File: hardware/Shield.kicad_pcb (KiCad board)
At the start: 2 copper layers, 29 parts, among them IC1 TP4056-42-ESOP8, P1 CONN_14_1, P2 CONN_14_2, SW1 JS202011SCQN

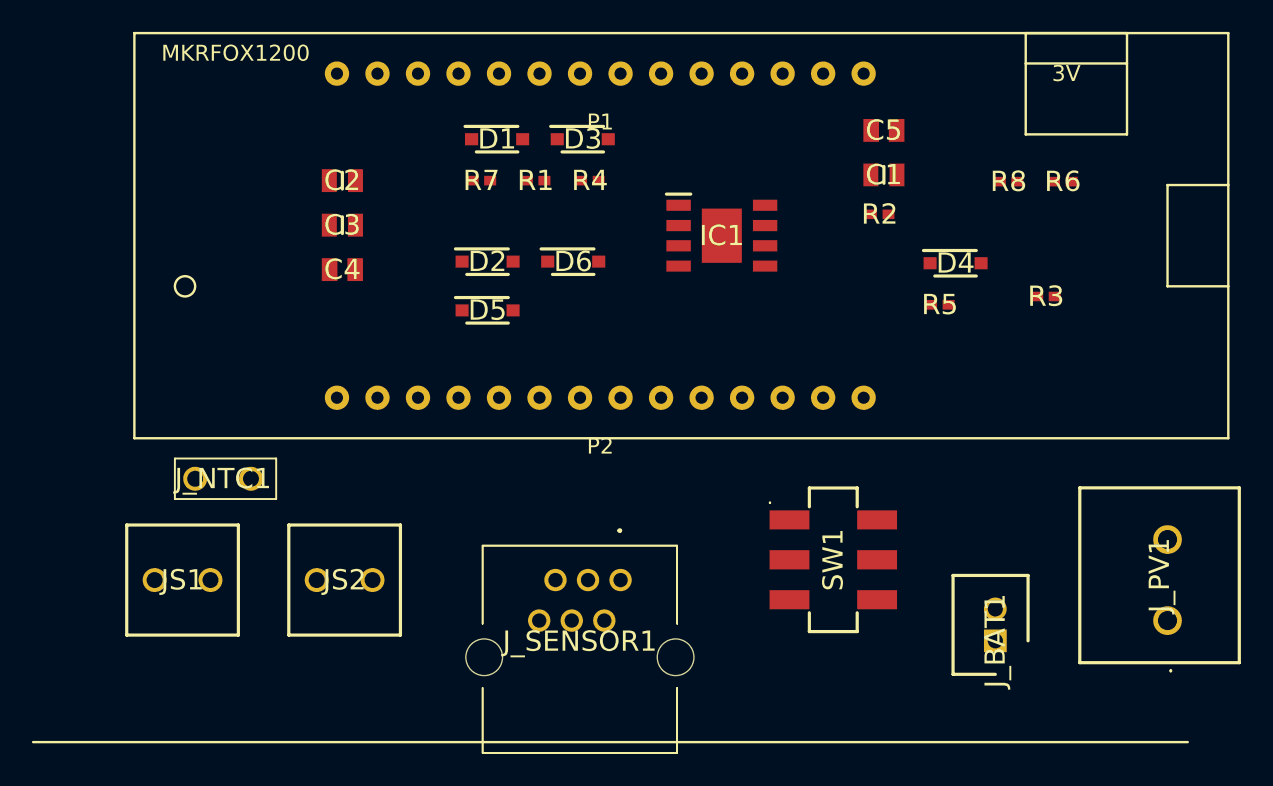
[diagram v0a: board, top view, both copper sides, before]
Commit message: completed PCB, DRC OK
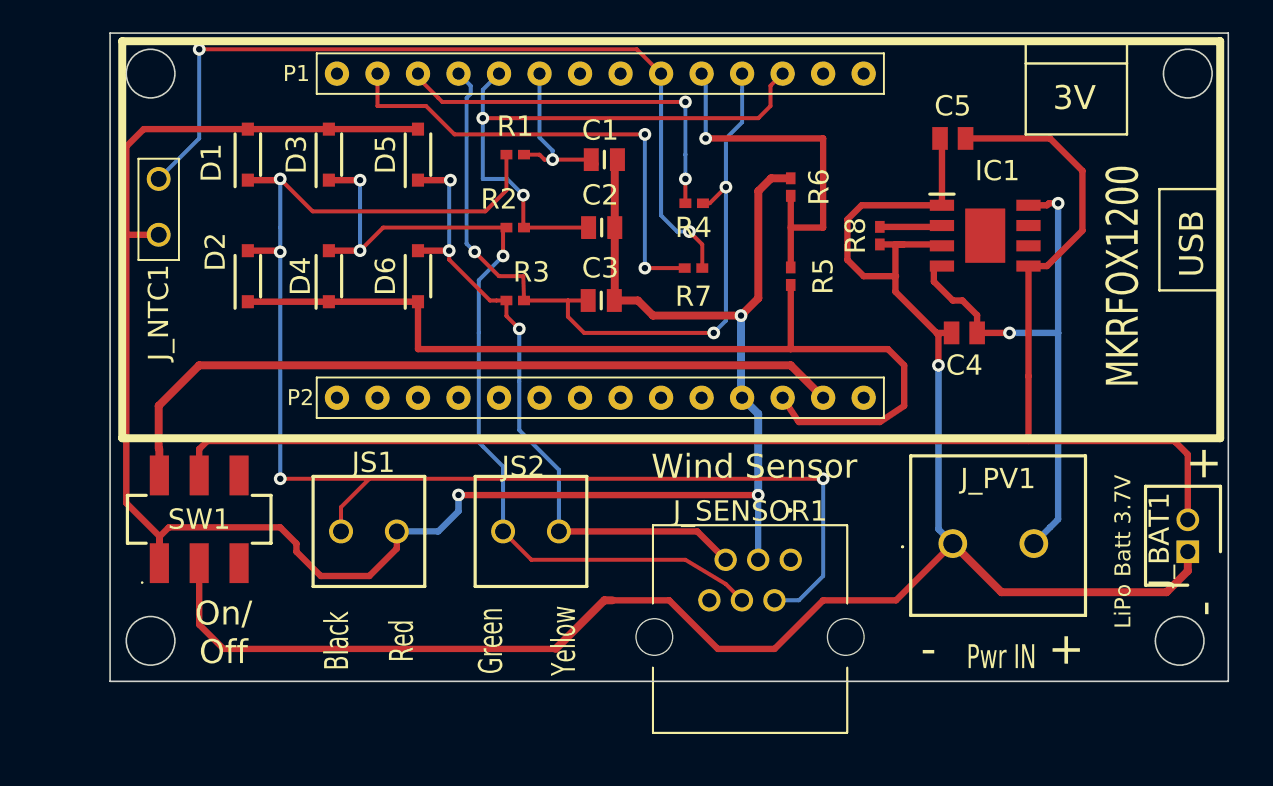
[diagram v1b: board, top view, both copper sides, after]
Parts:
- P1: footprint JLCPCB_FP:CONN14_FP -> JLCPCB_FP:CONN14_FP1
- P2: footprint JLCPCB_FP:CONN14_FP -> JLCPCB_FP:CONN14_FP2
- moved SW1 39.8 mm to (80.3, 96.5), turned to 0 degrees
- moved D4 39.3 mm to (88.4, 81.3), turned to 90 degrees
- moved C4 39.2 mm to (128.2, 84.8)
- moved R3 33.3 mm to (100.1, 82.8)
- moved R2 22.9 mm to (100.1, 78.2)
- moved J_NTC1 18.9 mm to (77.7, 75.2), turned to 270 degrees
- moved C1 17.6 mm to (105.7, 74.0), turned to 180 degrees
- moved R6 17.1 mm to (117.3, 75.7), turned to 90 degrees
- moved C3 16.9 mm to (105.5, 82.8), turned to 180 degrees
- moved C2 16.5 mm to (105.5, 78.2), turned to 180 degrees
- moved IC1 16.5 mm to (129.5, 78.7)
- moved D3 15.9 mm to (88.4, 73.7), turned to 90 degrees
- moved D1 15.7 mm to (83.3, 73.7), turned to 90 degrees
- moved D2 15.1 mm to (83.3, 81.3), turned to 90 degrees
- moved R7 14.4 mm to (111.3, 80.8)
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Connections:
- C1 pad 1: Net-(C1-Pad1) -> MGND
- C1 pad 2: Net-(C1-Pad2) -> D0
- C2 pad 1: Net-(C1-Pad1) -> MGND
- C2 pad 2: Net-(C2-Pad2) -> D1A1
- C3 pad 1: Net-(C1-Pad1) -> MGND
- C3 pad 2: Net-(C3-Pad2) -> D2A2
- C4 pad 2: Net-(C4-Pad2) -> VPV
- C5 pad 2: Net-(C5-Pad2) -> VBAT
- D1 pad 1: Net-(D1-Pad1) -> Wire1
- D1 pad 2: Net-(C1-Pad1) -> MGND
- D2 pad 1: Net-(D2-Pad1) -> VCC
- D2 pad 2: Net-(D1-Pad1) -> Wire1
- D3 pad 1: Net-(D3-Pad1) -> Wire3
- D3 pad 2: Net-(C1-Pad1) -> MGND
- D4 pad 1: Net-(D2-Pad1) -> VCC
- D4 pad 2: Net-(D3-Pad1) -> Wire3
- D5 pad 1: Net-(D5-Pad1) -> Wire4
- D5 pad 2: Net-(C1-Pad1) -> MGND
- D6 pad 1: Net-(D2-Pad1) -> VCC
- D6 pad 2: Net-(D5-Pad1) -> Wire4
- IC1 pad 4: Net-(C4-Pad2) -> VPV
- IC1 pad 5: Net-(C5-Pad2) -> VBAT
- IC1 pad 8: Net-(C4-Pad2) -> VPV
- JS1 pad 1: Net-(C1-Pad1) -> Wire1
- JS1 pad 2: Net-(D1-Pad1) -> MGND
- JS2 pad 1: Net-(D5-Pad1) -> Wire3
- JS2 pad 2: Net-(D3-Pad1) -> Wire4
- J_BAT1 pad 1: Net-(C5-Pad2) -> GND
- J_BAT1 pad 2: GND -> VBAT
- J_NTC1 pad 1: Net-(C1-Pad1) -> A4
- J_NTC1 pad 2: Net-(J_NTC1-Pad2) -> MGND
- J_PV1 pad 1: Net-(C4-Pad2) -> GND
- J_PV1 pad 2: GND -> VPV
- J_SENSOR1 pad 2: Net-(D1-Pad1) -> Wire1
- J_SENSOR1 pad 3: Net-(C1-Pad1) -> MGND
- J_SENSOR1 pad 4: Net-(D3-Pad1) -> Wire3
- J_SENSOR1 pad 5: Net-(D5-Pad1) -> Wire4
- P1 pad 1: Net-(P1-Pad1) -> D1A1
- P1 pad 2: Net-(P1-Pad2) -> D2A2
- P1 pad 3: Net-(C2-Pad2) -> D3
- P1 pad 4: Net-(C3-Pad2) -> D4
- P1 pad 5: Net-(P1-Pad5) -> (no net)
- P2 pad 10: Net-(P2-Pad10) -> (no net)
- P2 pad 11: Net-(P2-Pad11) -> (no net)
- P2 pad 12: Net-(P2-Pad12) -> (no net)
- P2 pad 13: Net-(P2-Pad13) -> (no net)
- P2 pad 14: Net-(P2-Pad14) -> (no net)
- P2 pad 6: Net-(P2-Pad6) -> (no net)
- P2 pad 7: Net-(P2-Pad7) -> (no net)
- P2 pad 8: Net-(P2-Pad8) -> (no net)
- P2 pad 9: Net-(P2-Pad9) -> (no net)
- R1 pad 1: Net-(D1-Pad1) -> Wire1
- R1 pad 2: Net-(C1-Pad2) -> D0
- R2 pad 1: Net-(D3-Pad1) -> Wire3
- R2 pad 2: Net-(C2-Pad2) -> D1A1
- R3 pad 1: Net-(D5-Pad1) -> Wire4
- R3 pad 2: Net-(C3-Pad2) -> D2A2
- R4 pad 1: Net-(C3-Pad2) -> D2A2
- R4 pad 2: Net-(P1-Pad12) -> D3
- R5 pad 1: Net-(D2-Pad1) -> VCC
- R5 pad 2: Net-(P1-Pad5) -> A3
- R6 pad 1: Net-(P1-Pad5) -> A3
- R6 pad 2: Net-(C1-Pad1) -> MGND
- R7 pad 1: Net-(P1-Pad13) -> D4
- R7 pad 2: Net-(J_NTC1-Pad2) -> A4
- SW1 pad 1: Net-(C1-Pad1) -> MGND
- SW1 pad 5: Net-(C5-Pad2) -> VBAT
- SW1 pad 6: Net-(P2-Pad2) -> VIN
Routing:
- net MGND: track 0.00 -> 135.7 mm, vias 0 -> 3
- net GND: track 0.00 -> 116.0 mm, vias 0 -> 1
- net VBAT: track 0.00 -> 95.5 mm
- net Wire1: track 0.00 -> 88.6 mm, vias 0 -> 4
- net VCC: track 0.00 -> 59.8 mm
- net Wire3: track 0.00 -> 55.2 mm, vias 0 -> 3
- net A4: track 0.00 -> 52.5 mm, vias 0 -> 2
- net D2A2: track 0.00 -> 50.5 mm, vias 0 -> 3
- net VIN: track 0.00 -> 47.9 mm
- net Wire4: track 0.00 -> 40.7 mm, vias 0 -> 3
- net D1A1: track 0.00 -> 36.8 mm, vias 0 -> 2
- net VPV: track 0.00 -> 34.6 mm, vias 0 -> 2
- net D4: track 0.00 -> 30.4 mm, vias 0 -> 2
- net D3: track 0.00 -> 24.0 mm, vias 0 -> 2
- net A3: track 0.00 -> 23.6 mm, vias 0 -> 1
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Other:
- board outline added: 70.1 x 40.6 mm
- net class PWR added: clearance 0.2, trace_width 0.5, via_dia 0.8, via_drill 0.4
- board text added: "+"
- board text added: "-"
- board text added: "Black"
- board text added: "Green"
- board text added: "LiPo Batt 3.7V"
- board text added: "MkrfoxWindShield"
- board text added: "On/ Off"
- board text added: "Pwr IN"
- board text added: "Red"
- board text added: "USB"
- board text added: "Wind Sensor"
- board text added: "Yellow"
